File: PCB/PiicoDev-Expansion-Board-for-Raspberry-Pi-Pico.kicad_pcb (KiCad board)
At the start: 2 copper layers, 50.4 x 51.4 mm, 33 parts, among them J1 PiicoDev, J2 JST PH, J3 , J4 , Q1 MOSFET P-CH, U1 TPS54302

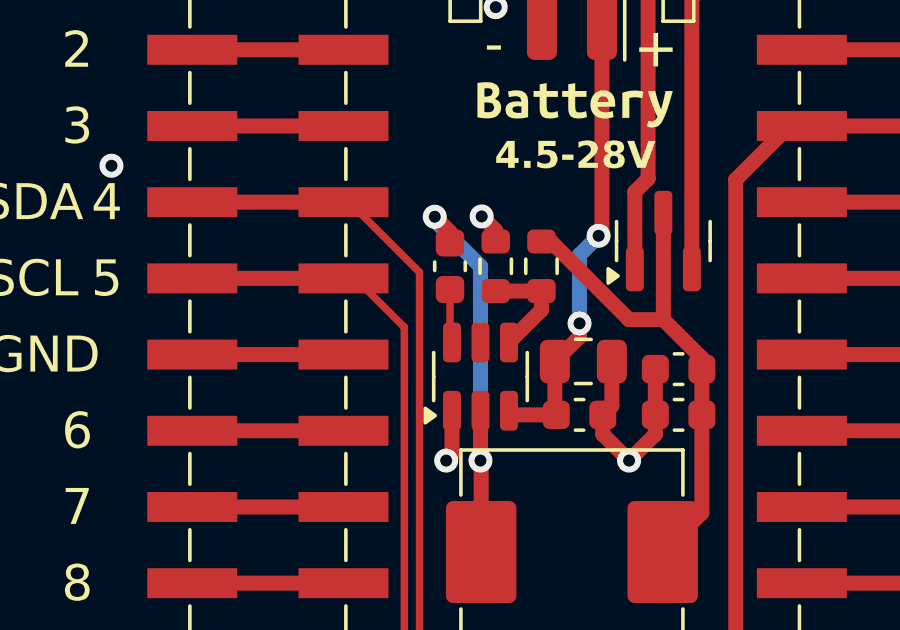
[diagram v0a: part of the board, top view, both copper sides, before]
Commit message: prototype production
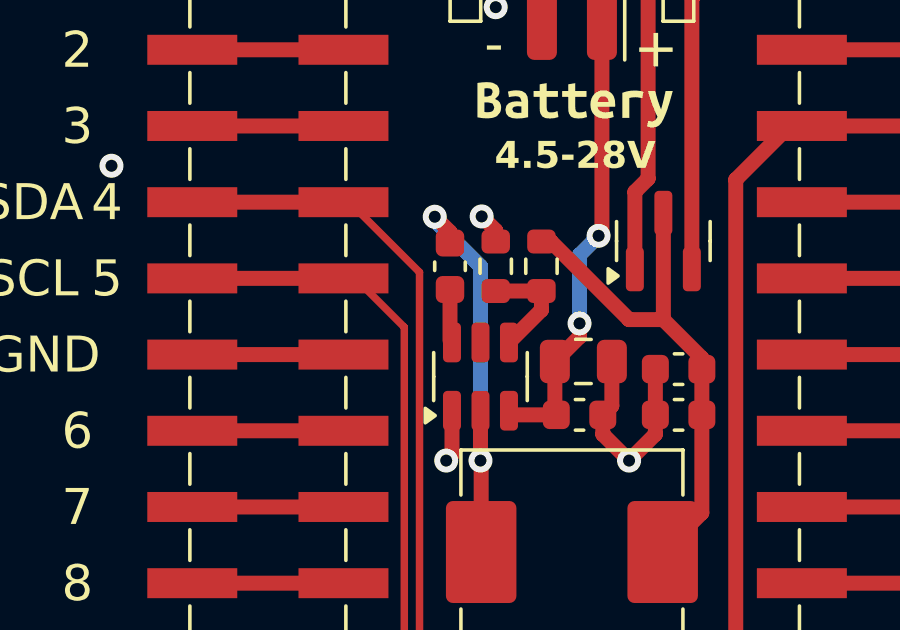
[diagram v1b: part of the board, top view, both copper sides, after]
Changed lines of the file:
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@@
 			)
 		)
-		(property "LCSC" "C2845363"
+		(property "LCSC" "C160404"
 			(at 0 0 0)
 			(unlocked yes)
@@
 		(sheetname "Root")
 		(sheetfile "PiicoDev-Expansion-Board-for-Raspberry-Pi-Pico.kicad_sch")
-		(attr exclude_from_pos_files)
+		(attr exclude_from_pos_files exclude_from_bom)
 		(fp_circle
 			(center 0 0)
@@
 		)
 		(fp_text user "${REFERENCE}"
-			(at 0 0 360)
+			(at 0 0 0)
 			(layer "F.Fab")
 			(hide yes)
@@
 		(sheetname "Root")
 		(sheetfile "PiicoDev-Expansion-Board-for-Raspberry-Pi-Pico.kicad_sch")
-		(attr exclude_from_pos_files)
+		(attr exclude_from_pos_files exclude_from_bom)
 		(fp_circle
 			(center 0 0)
@@
 		(sheetname "Root")
 		(sheetfile "PiicoDev-Expansion-Board-for-Raspberry-Pi-Pico.kicad_sch")
-		(attr exclude_from_pos_files)
+		(attr exclude_from_pos_files exclude_from_bom)
 		(fp_circle
 			(center 0 0)
@@
 		(sheetname "Root")
 		(sheetfile "PiicoDev-Expansion-Board-for-Raspberry-Pi-Pico.kicad_sch")
-		(attr exclude_from_pos_files)
+		(attr exclude_from_pos_files exclude_from_bom)
 		(fp_circle
 			(center 0 0)
@@
 		(sheetname "Root")
 		(sheetfile "PiicoDev-Expansion-Board-for-Raspberry-Pi-Pico.kicad_sch")
-		(attr exclude_from_pos_files)
+		(attr exclude_from_pos_files exclude_from_bom)
 		(fp_line
 			(start -0.7 1)
@@
 		)
 		(property "Value" "I2C"
-			(at 0 1.9 360)
+			(at 0 1.9 0)
 			(layer "F.Fab")
 			(effects
@@
 		)
 		(property "Footprint" "CoreElectronics_Components:SolderJumper-3_P1.3mm_Closed_RoundedPad1.0x1.5mm"
-			(at 0 0 360)
+			(at 0 0 0)
 			(layer "B.Fab")
 			(hide yes)
@@
 		)
 		(property "Datasheet" ""
-			(at 0 0 360)
+			(at 0 0 0)
 			(layer "B.Fab")
 			(hide yes)
@@
 		)
 		(property "Description" ""
-			(at 0 0 360)
+			(at 0 0 0)
 			(layer "B.Fab")
 			(hide yes)
@@
 		(sheetname "Root")
 		(sheetfile "PiicoDev-Expansion-Board-for-Raspberry-Pi-Pico.kicad_sch")
-		(attr exclude_from_pos_files)
+		(attr exclude_from_pos_files exclude_from_bom)
 		(net_tie_pad_groups "1, 2, 3")
 		(fp_line
@@
 		)
 		(property "Value" "0.1uF"
-			(at 0 1.43 360)
+			(at 0 1.43 0)
 			(layer "F.Fab")
 			(effects
@@
 		)
 		(fp_text user "${REFERENCE}"
-			(at 0 0 360)
+			(at 0 0 0)
 			(layer "F.Fab")
 			(effects
@@
 		)
 		(property "Value" "10uF"
-			(at 0 1.68 360)
+			(at 0 1.68 0)
 			(layer "F.Fab")
 			(effects
@@
 		)
 		(fp_text user "${REFERENCE}"
-			(at 0 0 360)
+			(at 0 0 0)
 			(layer "F.Fab")
 			(effects
@@
 		)
 		(property "Value" "22uF"
-			(at 0 1.43 360)
+			(at 0 1.43 0)
 			(layer "F.Fab")
 			(effects
@@
 		)
 		(fp_text user "${REFERENCE}"
-			(at 0 0 360)
+			(at 0 0 0)
 			(layer "F.Fab")
 			(effects
@@
 		)
 		(property "Value" "22uF"
-			(at 0 1.43 360)
+			(at 0 1.43 0)
 			(layer "F.Fab")
 			(effects
@@
 		)
 		(fp_text user "${REFERENCE}"
-			(at 0 0 360)
+			(at 0 0 0)
 			(layer "F.Fab")
 			(effects
@@
 		(sheetname "Root")
 		(sheetfile "PiicoDev-Expansion-Board-for-Raspberry-Pi-Pico.kicad_sch")
-		(attr exclude_from_pos_files)
+		(attr exclude_from_pos_files exclude_from_bom)
 		(fp_line
 			(start 0.7 -1)
@@
 		(start 136.771 90.071)
 		(end 136.771 91.77)
-		(width 0.25)
+		(width 0.5)
 		(layer "F.Cu")
 		(net 40)
